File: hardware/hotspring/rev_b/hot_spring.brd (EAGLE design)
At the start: 32.5 x 13 mm, 27 parts, among them J1 GECKO_POWER_SUPPLY_CONN, J2 JUMPER-31-2, Q1 MOSFET-NCHANNELSMD, Q2 MOSFET-NCHANNELSMD, Q3 DUAL_MOSFET_NP, T1 LPR6235-752SMR, T2 LPR6235-752SMR, U1 LTC3109EUF

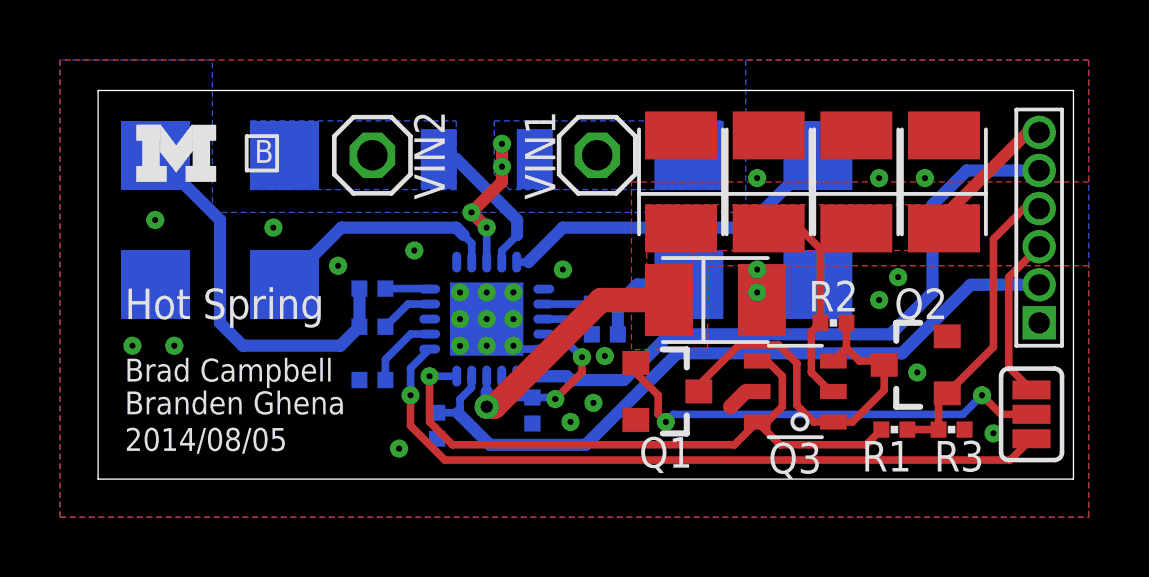
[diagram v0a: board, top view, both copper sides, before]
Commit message: hot spring updates
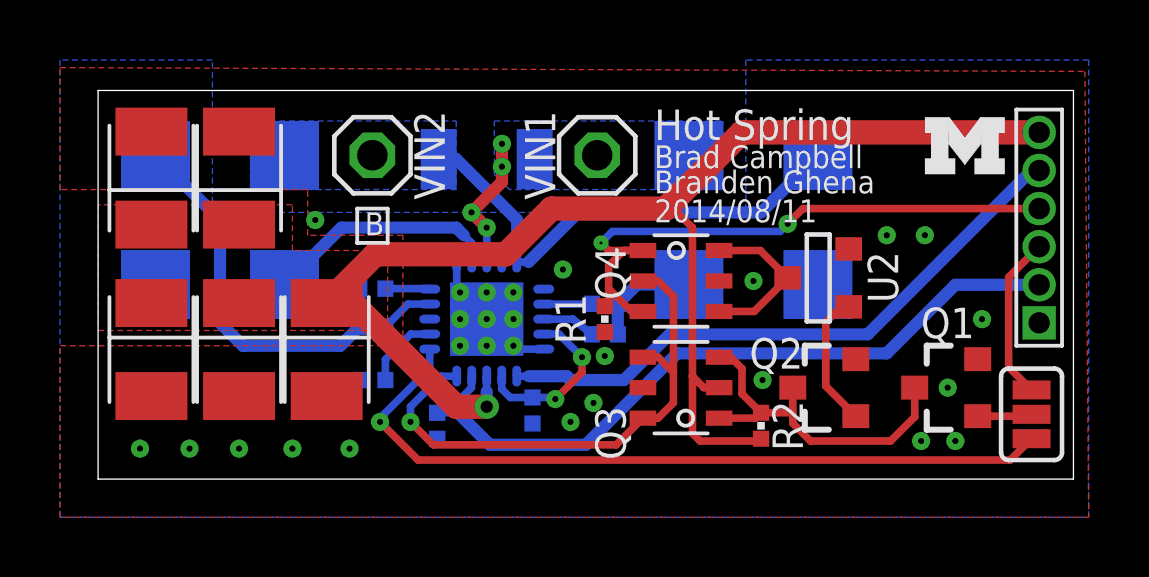
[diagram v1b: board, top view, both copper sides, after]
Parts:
- removed R3: 500k, passives:0402_RES
- added Q4: DUAL_MOSFET_NP, fets:TSOP-6
- added U2: TC54VC2102ECB713, chips:SOT-23
- R1: value 250k -> 100k
- moved LOGO1 26.3 mm to (27.6, 10.2)
- moved C11 21.3 mm to (1.78, 4.32), turned to 0 degrees
- moved C10 21.3 mm to (4.70, 4.32), turned to 0 degrees
- moved C9 21.3 mm to (7.62, 4.32), turned to 0 degrees
- moved C13 19.2 mm to (1.78, 10.0), turned to 180 degrees
- moved C12 14.7 mm to (4.70, 10.0)
- moved R1 10.3 mm to (16.9, 5.33), turned to 90 degrees
- moved Q1 9.40 mm to (28.3, 3.05), turned to 90 degrees
- moved R2 4.19 mm to (22.1, 1.78), turned to 270 degrees
- moved Q3 3.81 mm to (19.4, 3.05)
- moved Q2 3.14 mm to (24.3, 3.05)
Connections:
- new net N$13: Q2.1, U2.1
- new net N$5: Q4.4, Q4.6, U2.3
- net GND: now also Q4.5, R1.1, U2.2; no longer R3.1
- net SHUTDOWN: now also Q4.1, Q4.3, R1.2; no longer Q2.1, R1.1, R3.2
- net VOUT2_EN: now also Q4.2; no longer R1.2
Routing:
- net VOUT: track 20.6 -> 45.3 mm
- net N$11: track 15.2 -> 1.82 mm, vias 2 -> 0
- net SHUTDOWN: track 10.1 -> 20.8 mm, vias 0 -> 2
- net N$5: track 0.00 -> 5.41 mm
- net N$13: track 0.00 -> 4.50 mm
- net VOUT2_EN: track 21.8 -> 18.1 mm
- net VSTORE: track 22.1 -> 20.4 mm
- net PGOOD: track 24.3 -> 25.7 mm
- net N$14: track 13.1 -> 12.0 mm
- net GND: track 2.16 -> 2.11 mm, vias 29 -> 27
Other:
- board text added: "2014/08/11"
- board text removed: "2014/08/05"

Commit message: squall routed
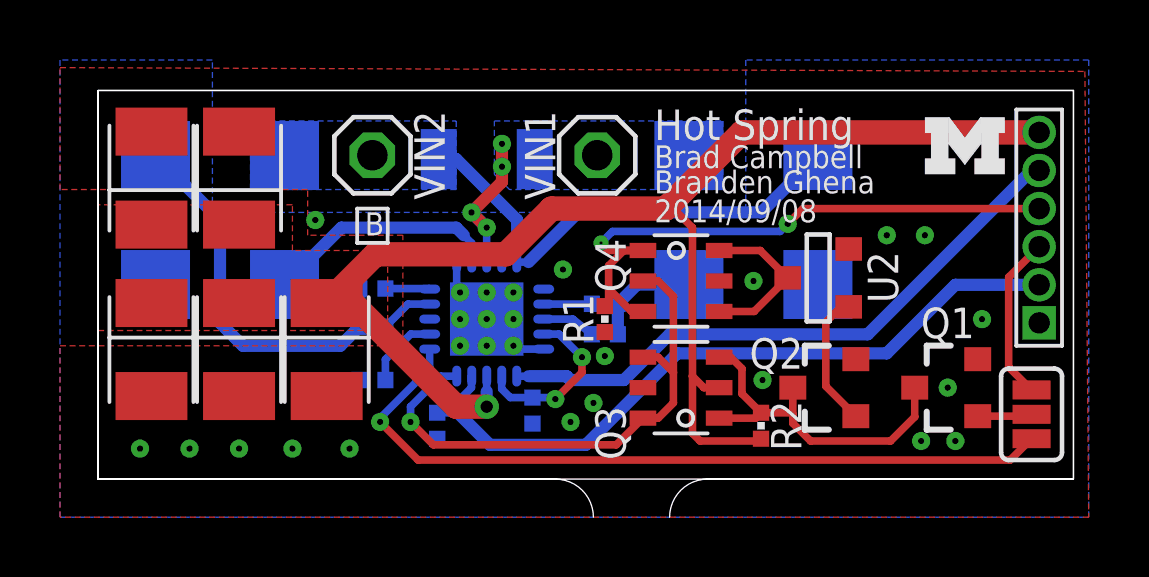
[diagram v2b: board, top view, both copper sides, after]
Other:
- board size 32.5 x 13 mm -> 32.5 x 14.2 mm
- board text added: "2014/09/08"
- board text removed: "2014/08/11"
